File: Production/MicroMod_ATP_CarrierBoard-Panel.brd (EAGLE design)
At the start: 200.9 x 126 mm, 877 parts, among them J19 QWIIC_RIGHT_ANGLE, J2 JTAG, J20 QWIIC_RIGHT_ANGLE, J21 1X04_SMD_STRAIGHT_COMBO, J27 MICROMOD-2222-C, J28 USB_A_SMT_FEMALE, J34 QWIIC_RIGHT_ANGLE, J35 QWIIC_RIGHT_ANGLE, J37 1X04_SMD_STRAIGHT_COMBO, J4 USB_A_SMT_FEMALE, J40 1X04_SMD_STRAIGHT_COMBO, J50 JTAG, J51 MICROMOD-2222-C, J52 USB_A_SMT_FEMALE, J58 QWIIC_RIGHT_ANGLE, J59 QWIIC_RIGHT_ANGLE, J6 MICROMOD-2222-C, J61 1X04_SMD_STRAIGHT_COMBO, J64 1X04_SMD_STRAIGHT_COMBO, J7 JTAG, J74 JTAG, J75 MICROMOD-2222-C, J76 USB_A_SMT_FEMALE, J8 1X04_SMD_STRAIGHT_COMBO, J82 QWIIC_RIGHT_ANGLE, J83 QWIIC_RIGHT_ANGLE, J85 1X04_SMD_STRAIGHT_COMBO, J88 1X04_SMD_STRAIGHT_COMBO, U1 AP7361C-33, U2 AP7361C-33, U3 AP7361C-33, U5 AP7361C-33

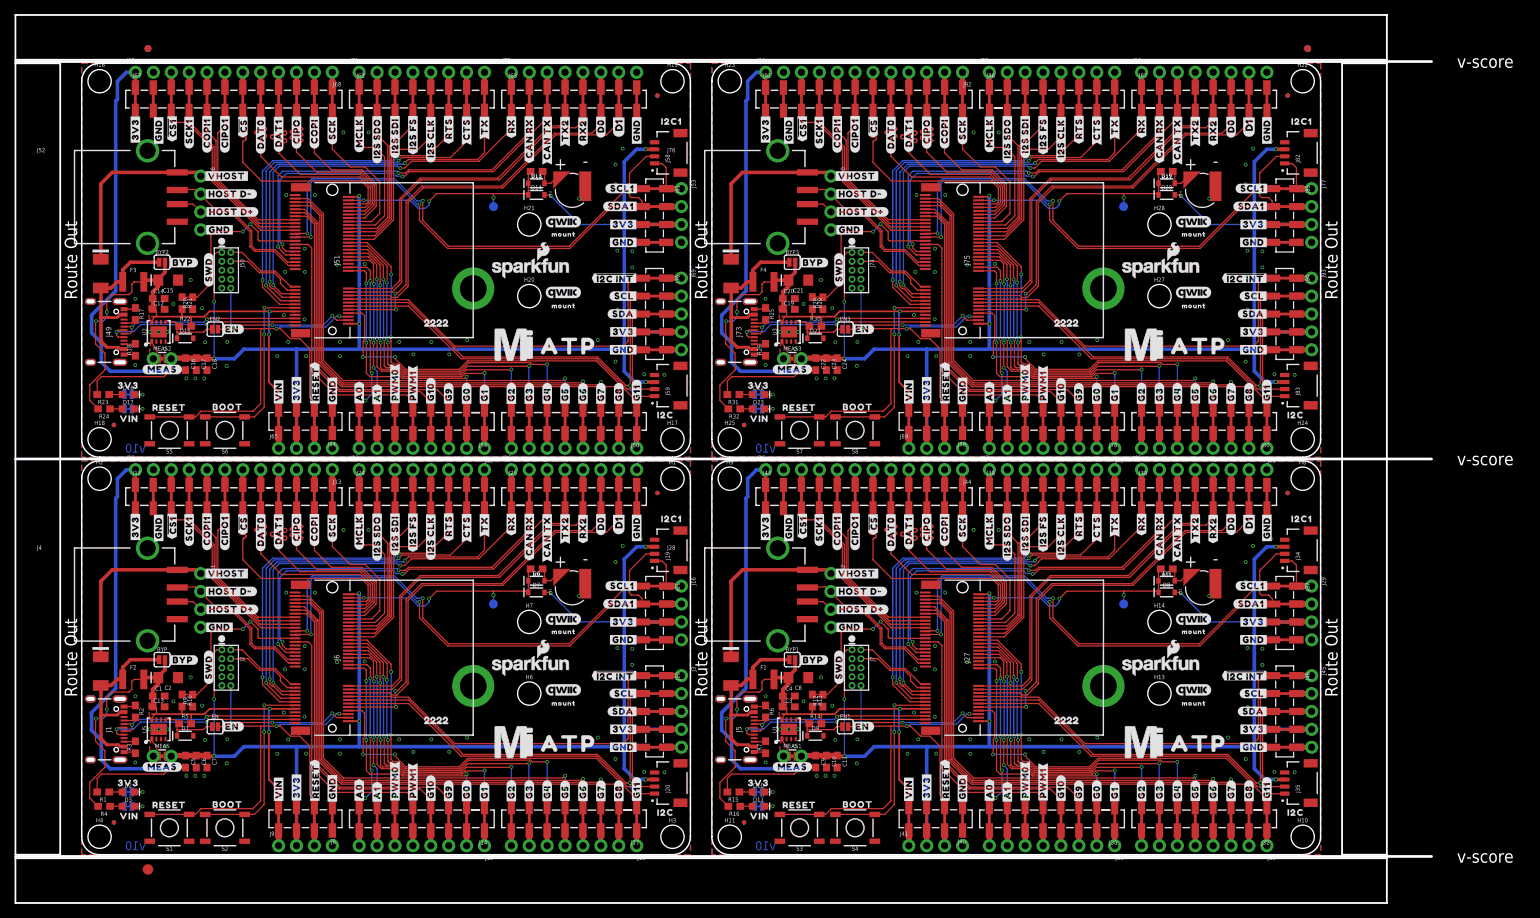
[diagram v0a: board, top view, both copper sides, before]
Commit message: Updates production files
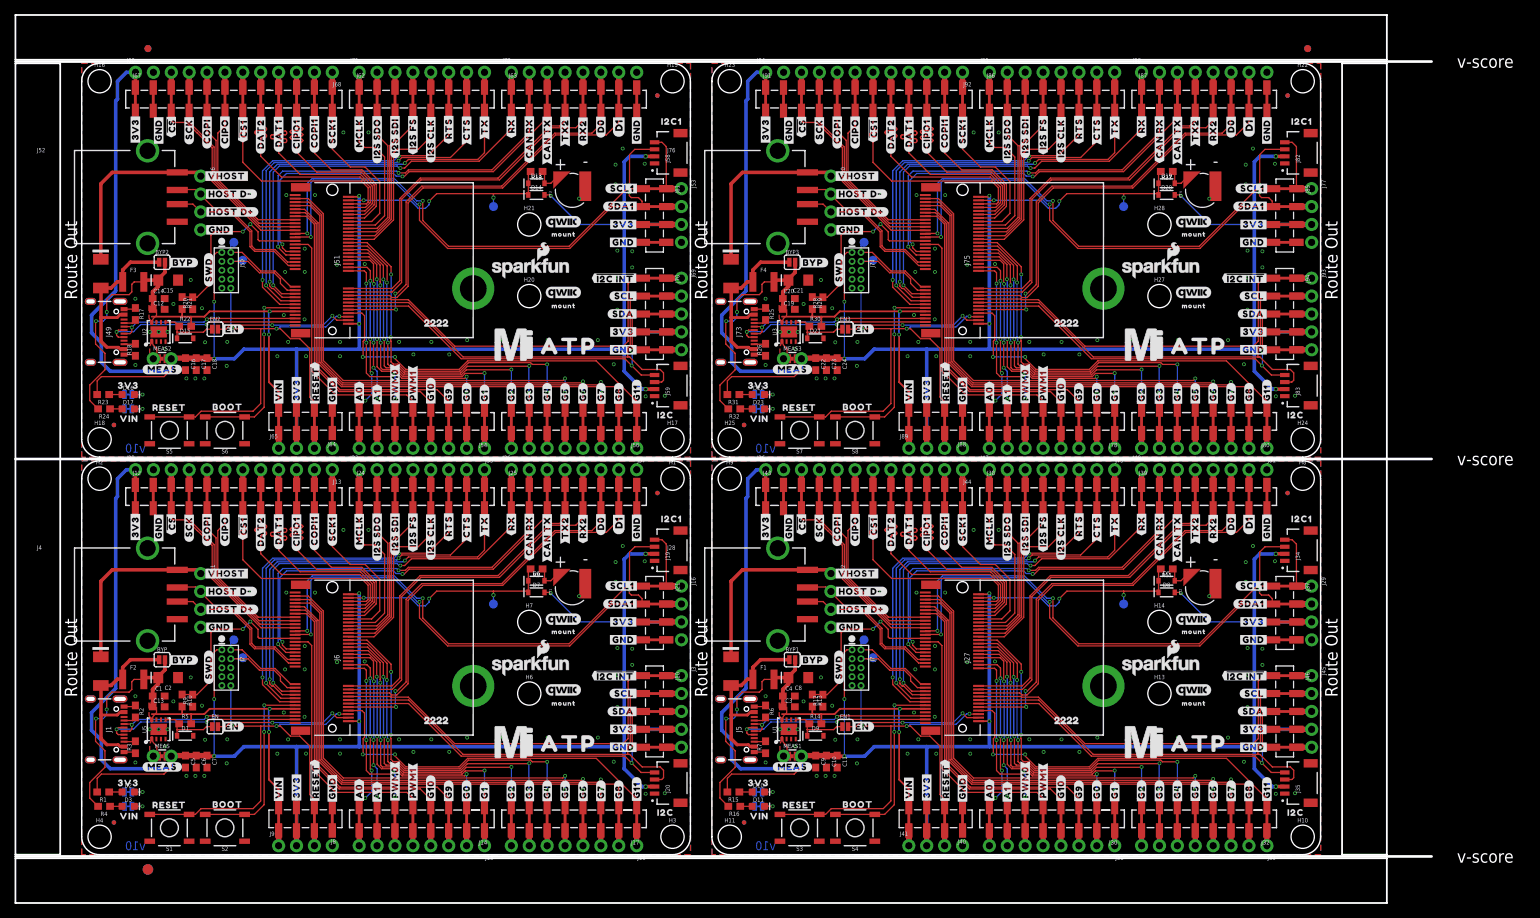
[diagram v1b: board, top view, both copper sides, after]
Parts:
- added E$6: (no value), SparkFun-Retired:FIDUCIAL-1.5X3
- added TP10, TP11, TP12, TP5, TP6, TP7, TP8, TP9: TEST-POINT3X5, SparkFun-Connectors:PAD.03X.05
- U$130: device buzzard_labels (9):22229 -> headtop:#CAN_RX#9
- U$147: device headtop:#CAN_RX#9 -> alc:#CIPO#5178038
- U$190, U$335, U$480: device headtop:#DAT1#4 -> headers_dup:#RX2#3
- U$191, U$336, U$481: device headtop:#DAT0#4 -> headers_dup:#TX2#2
- U$192, U$337, U$482: device headers_dup:#RX2#3 -> headers_dup:#SCL1#3
- U$193, U$338, U$483: device headers_dup:#TX2#2 -> headers_dup:#SDA1#3
- U$194, U$339, U$484: device headers_dup:#SCL1#3 -> headers_dup:#SCK1#2
- U$195, U$340, U$485: device headers_dup:#SDA1#3 -> headers_dup:VIN3
- U$196, U$341, U$486: device headers_dup:#SCK1#2 -> headers_dup:3V34
- U$197, U$342, U$487: device headers_dup:VIN3 -> power:#3V3#1
- U$198, U$343, U$488: device headers_dup:3V34 -> power:#3V3#1
- U$20: device headers_dup:##CS1##2 -> alc:##CS1##5178039
- U$201, U$346, U$491: device power:#3V3#1 -> headers_dup:ATP0
- U$202, U$347, U$492: device power:#3V3#1 -> headers_dup:I2C4
- U$203, U$348, U$493: device headers_dup:ATP0 -> headers_dup:I2C14
- U$204, U$349, U$494: device headers_dup:I2C4 -> headers_dup:ATP_CARRIER_BOARD1
- U$205, U$350, U$495: device headers_dup:I2C14 -> headers_dup:#COPI1#2
- U$206, U$351, U$496: device headers_dup:ATP_CARRIER_BOARD1 -> power:##RESET##7
- U$207, U$352, U$497: device fl1:##CS1##0 -> headtop:##CS##0
- U$208, U$353, U$498: device headers_dup:#CIPO1#2 -> fl1:#COPI1#2
- U$209, U$354, U$499: device headers_dup:#COPI1#2 -> fl1:#RX2#3
- U$210, U$355, U$500: device headers_dup:##CS1##2 -> fl1:#SCK1#2
- U$211, U$356, U$501: device power:##RESET##7 -> fl1:#SCL1#3
- U$212, U$357, U$502: device headtop:##CS##0 -> fl1:#SDA1#3
- U$213, U$358, U$503: device fl1:#CIPO1#2 -> fl1:#TX2#2
- U$214, U$359, U$504: device fl1:#COPI1#2 -> fl2:#DAT2#5
- U$215, U$360, U$505: device fl1:#RX2#3 -> fl2:#DAT1#5
- U$216, U$361, U$506: device fl1:#SCK1#2 -> fl2:#COPI#4
- U$217, U$362, U$507: device fl1:#SCL1#3 -> fl2:#SCK#4
- U$218, U$363, U$508: device fl1:#SDA1#3 -> fl2:#MCLK#6
- U$219, U$364, U$509: device fl1:#TX2#2 -> fl2:#I2S_FS#7
- U$220, U$365, U$510: device fl2:##CS##DAT3#0 -> fl2:#I2S_CLK#7
- U$221, U$366, U$511: device fl2:#DAT2#5 -> fl2:#RTS#7
- U$222, U$367, U$512: device fl2:#DAT1#5 -> fl2:#CTS#8
- U$223, U$368, U$513: device fl2:#COPI#4 -> fl2:#TX#9
- U$224, U$369, U$514: device fl2:#SCK#4 -> fl2:#RX#10
- U$225, U$370, U$515: device fl2:#MCLK#6 -> fl2:#CAN_RX#10
- U$226, U$371, U$516: device fl2:#I2S_FS#7 -> fl2:#CAN_TX#10
- U$227, U$372, U$517: device fl2:#I2S_CLK#7 -> fl4:#D0#0
- U$228, U$373, U$518: device fl2:#RTS#7 -> fl3:#GND#0
- U$229, U$374, U$519: device fl2:#CTS#8 -> fl3:#GND#0
- U$230, U$375, U$520: device fl2:#TX#9 -> fl3:#GND#0
- U$231, U$376, U$521: device fl2:#RX#10 -> fl3:#GND#0
- U$232, U$377, U$522: device fl2:#CAN_RX#10 -> fl3:#GND#0
- U$233, U$378, U$523: device fl2:#CAN_TX#10 -> fl3:#GND#0
- U$234, U$379, U$524: device fl4:#D0#0 -> fl3:#3V3#1
- U$235, U$380, U$525: device fl3:#GND#0 -> fl3:#3V3#1
- U$236, U$381, U$526: device fl3:#GND#0 -> fl3:#SDA#4
- U$237, U$382, U$527: device fl3:#GND#0 -> fl3:#SCL#5
- U$238, U$383, U$528: device fl3:#GND#0 -> fl2:##I2C_INT##10
- U$239, U$384, U$529: device fl3:#GND#0 -> fl4:#G11#10
- U$240, U$385, U$530: device fl3:#GND#0 -> fl4:#G8#8
- U$241, U$386, U$531: device fl3:#3V3#1 -> fl4:#G7#7
- U$242, U$387, U$532: device fl3:#3V3#1 -> fl4:#G6#6
- U$243, U$388, U$533: device fl3:#SDA#4 -> fl4:#G5#5
- U$244, U$389, U$534: device fl3:#SCL#5 -> fl4:#G4#4
- U$245, U$390, U$535: device fl2:##I2C_INT##10 -> fl4:#G3#3
- U$246, U$391, U$536: device fl4:#G11#10 -> fl4:#G2#2
- U$247, U$392, U$537: device fl4:#G8#8 -> fl4:#G1#2
- U$248, U$393, U$538: device fl4:#G7#7 -> fl4:#G0#2
- U$249, U$394, U$539: device fl4:#G6#6 -> fl4:#PWM0#10
- U$250, U$395, U$540: device fl4:#G5#5 -> fl4:#PWM1#10
- U$251, U$396, U$541: device fl4:#G4#4 -> fl4:#A0#10
- U$252, U$397, U$542: device fl4:#G3#3 -> fl4:#A1#10
- U$253, U$398, U$543: device fl4:#G2#2 -> fl3:##RESET##7
- U$254, U$399, U$544: device fl4:#G1#2 -> fl3:#3V3#1
- U$255, U$400, U$545: device fl4:#G0#2 -> fl3:#VIN#6
- U$256, U$401, U$546: device fl4:#PWM0#10 -> fl3:#HOST_D##9
- U$257, U$402, U$547: device fl4:#PWM1#10 -> fl3:#HOST_D##10
- U$258, U$403, U$548: device fl4:#A0#10 -> fl3:#SWD#10
- U$259, U$404, U$549: device fl4:#A1#10 -> fl3:#MEAS#10
- U$260, U$405, U$550: device fl3:##RESET##7 -> fl3:#VIN_LED#10
- U$261, U$406, U$551: device fl3:#3V3#1 -> fl3:#3V3_LED#10
- U$262, U$407, U$552: device fl3:#VIN#6 -> fl4:#G9#ADC##CAM_HSYNC#9
- U$263, U$408, U$553: device fl3:#HOST_D##9 -> fl4:#G10#ADC##CAM_VSYNC#10
- U$264, U$409, U$554: device fl3:#HOST_D##10 -> fl2:#I2S_SDI#CAM_PCLK#7
- U$265, U$410, U$555: device fl3:#SWD#10 -> fl2:#I2S_SDO#CAM_MCLK#7
- U$266, U$411, U$556: device fl3:#MEAS#10 -> fl3:#3V3#1
- U$267, U$412, U$557: device fl3:#VIN_LED#10 -> headtop:#SCK#2
- U$268, U$413, U$558: device fl3:#3V3_LED#10 -> power:#GND#0
- U$269, U$414, U$559: device fl4:#G9#ADC##CAM_HSYNC#9 -> power:#GND#0
- U$270, U$415, U$560: device fl4:#G10#ADC##CAM_VSYNC#10 -> power:#GND#0
- U$271, U$416, U$561: device fl2:#I2S_SDI#CAM_PCLK#7 -> headtop:##I2C_INT##10
- U$272, U$417, U$562: device fl2:#I2S_SDO#CAM_MCLK#7 -> D1:D10
- U$273, U$418, U$563: device fl3:#3V3#1 -> SparkFun-MicroMod:MICROMOD_MI_LOGO_1
- U$274, U$419, U$564: device headtop:#SCK#2 -> headtop:MOUNT10
- U$275, U$276, U$277, U$420, U$421, U$422, U$565, U$566, U$567: device power:#GND#0 -> headtop:MOUNT10
- U$278, U$423, U$568: device headtop:##I2C_INT##10 -> SparkFun-MicroMod:MICROMOD_LOGO_1
- U$279, U$424, U$569: device D1:D10 -> D1_again:D10
- U$280, U$425, U$570: device SparkFun-MicroMod:MICROMOD_MI_LOGO_1 -> output:#EN#0
- U$281, U$282, U$426, U$427, U$571, U$572: device headtop:MOUNT10 -> output:#VHOST#0
- U$283, U$428, U$573: device headtop:MOUNT10 -> alc:##CS##5178037
- U$284, U$429, U$574: device headtop:MOUNT10 -> alc:##CS1##DAT3#5178037
- U$285, U$430, U$575: device SparkFun-MicroMod:MICROMOD_LOGO_1 -> alc:#CIPO#5178038
- U$286, U$431, U$576: device fl2:#CIPO#DAT0#6 -> alc:##CS1##5178039
- U$287, U$432, U$577: device D1_again:D10 -> alc:#DAT1#5178039
- U$288, U$433, U$578: device output:#EN#0 -> alc:#DAT2#5178039
- U$289, U$434, U$579: device output:#VHOST#0 -> alc:#CIPO1#5178039
- U$290, U$435, U$580: device output:#VHOST#0 -> alc:##CIPO1##DAT0#5178038
- U$36: device fl1:##CS1##0 -> alc:#DAT1#5178039
- U$53: device headtop:#DAT1#4 -> alc:#DAT2#5178039
- U$54: device headtop:#DAT0#4 -> alc:#CIPO1#5178039
- U$56: device headers_dup:#CIPO1#2 -> alc:##CIPO1##DAT0#5178038
- U$74: device fl1:#CIPO1#2 -> buzzard_labels (9):22229
- U$81: device fl2:##CS##DAT3#0 -> alc:##CS##5178037
- U$84: device fl2:#CIPO#DAT0#6 -> alc:##CS1##DAT3#5178037
- moved U$147 132.7 mm to (20.3, 51.7), flipped to the bottom, turned to 270 degrees
- moved TP2 126.3 mm to (21.6, 30.5)
- moved U$74 121.1 mm to (137.0, 19.1), flipped to the top, turned to 0 degrees
- moved U$347 85.4 mm to (82.8, 62.4), turned to 0 degrees
- moved U$202 85.4 mm to (172.2, 5.97), turned to 0 degrees
- moved U$492 85.4 mm to (172.2, 62.4), turned to 0 degrees
- moved U$239 83.9 mm to (168.1, 3.56)
- moved U$384 83.9 mm to (78.7, 59.9)
- moved U$529 83.9 mm to (168.1, 59.9)
- moved U$195 76.0 mm to (96.1, 5.46)
- moved U$340 76.0 mm to (6.73, 61.8)
- moved U$485 76.0 mm to (96.1, 61.8)
- moved U$200 74.9 mm to (97.0, 46.5), turned to 90 degrees
- moved U$345 74.9 mm to (7.62, 102.9), turned to 90 degrees
- moved U$490 74.9 mm to (97.0, 102.9), turned to 90 degrees
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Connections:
- net !CS!/DAT1 renamed !CS1!/DAT1
- net !CS!/DAT2 renamed !CS1!/DAT2
- net !CS!/DAT3 renamed !CS1!/DAT3
- net !CS!/DAT4 renamed !CS1!/DAT4
- net !CS1 renamed !CS!
- net !CS2 renamed !CS!1
- net !CS3 renamed !CS!2
- net !CS4 renamed !CS!3
- net CIPO/DAT0 renamed CIPO1/DAT0
- net CIPO/DAT1 renamed CIPO1/DAT1
- net CIPO/DAT2 renamed CIPO1/DAT2
- net CIPO/DAT3 renamed CIPO1/DAT3
- removed net CIPO4: J75.61, J91.6, J92.7
- new net CIPO: J12.6, J13.7, J6.61
- net 3.3V: now also J19.2, J20.2; no longer J19.3, J20.3
- net 3.3V1: now also J34.2, J35.2; no longer J34.3, J35.3
- net 3.3V2: now also J58.2, J59.2; no longer J58.3, J59.3
- net 3.3V3: now also J82.2, J83.2; no longer J82.3, J83.3
- net CIPO1: now also J27.61, J43.6, J44.7; no longer J12.6, J13.7, J6.61
- net CIPO2: now also J51.61, J67.6, J68.7; no longer J27.61, J43.6, J44.7
- net CIPO3: now also J75.61, J91.6, J92.7; no longer J51.61, J67.6, J68.7
- net COPI: now also J12.5, J13.8, J6.59; no longer J12.11, J13.2, J6.62
- net COPI1: now also J12.11, J13.2, J6.62; no longer J12.5, J13.8, J6.59
- net COPI2: now also J27.59, J43.5, J44.8; no longer J27.62, J43.11, J44.2
- net COPI3: now also J27.62, J43.11, J44.2; no longer J27.59, J43.5, J44.8
- net COPI4: now also J51.59, J67.5, J68.8; no longer J51.62, J67.11, J68.2
- net COPI5: now also J51.62, J67.11, J68.2; no longer J51.59, J67.5, J68.8
- net COPI6: now also J75.59, J91.5, J92.8; no longer J75.62, J91.11, J92.2
- net COPI7: now also J75.62, J91.11, J92.2; no longer J75.59, J91.5, J92.8
- net GND: now also J19.1, J20.1; no longer J19.4, J20.4
- net GND1: now also J34.1, J35.1; no longer J34.4, J35.4
- net GND2: now also J58.1, J59.1; no longer J58.4, J59.4
- net GND3: now also J82.1, J83.1; no longer J82.4, J83.4
- net RTC_3V1: now also TP4.P$1; no longer TP2.P$1
- net RTC_3V2: now also TP7.P$1; no longer TP3.P$1
- net RTC_3V3: now also TP10.P$1; no longer TP4.P$1
- net SCK: now also J12.4, J22.4, J6.57; no longer J12.12, J13.1, J6.60
- net SCK1: now also J12.12, J13.1, J6.60; no longer J12.4, J22.4, J6.57
- net SCK2: now also J27.57, J36.4, J43.4; no longer J27.60, J43.12, J44.1
- net SCK3: now also J27.60, J43.12, J44.1; no longer J27.57, J36.4, J43.4
- net SCK4: now also J51.57, J60.4, J67.4; no longer J51.60, J67.12, J68.1
- net SCK5: now also J51.60, J67.12, J68.1; no longer J51.57, J60.4, J67.4
- net SCK6: now also J75.57, J84.4, J91.4; no longer J75.60, J91.12, J92.1
- net SCK7: now also J75.60, J91.12, J92.1; no longer J75.57, J84.4, J91.4
- net SCL: now also J20.3; no longer J20.1
- net SCL1: now also J19.4; no longer J19.1
- net SCL2: now also J35.3; no longer J35.1
- net SCL3: now also J34.4; no longer J34.1
- net SCL4: now also J59.3; no longer J59.1
- net SCL5: now also J58.4; no longer J58.1
- net SCL6: now also J83.3; no longer J83.1
- net SCL7: now also J82.4; no longer J82.1
- net SDA: now also J20.4; no longer J20.2
- net SDA1: now also J19.3; no longer J19.2
- net SDA2: now also J35.4; no longer J35.2
- net SDA3: now also J34.3; no longer J34.2
- net SDA4: now also J59.4; no longer J59.2
- net SDA5: now also J58.3; no longer J58.2
- net SDA6: now also J83.4; no longer J83.2
- net SDA7: now also J82.3; no longer J82.2
- net SWDCK: now also TP3.P$1
- net SWDCK1: now also TP6.P$1
- net SWDCK2: now also TP9.P$1
- net SWDCK3: now also TP12.P$1
- net SWDIO: now also TP2.P$1
- net SWDIO1: now also TP5.P$1
- net SWDIO2: now also TP8.P$1
- net SWDIO3: now also TP11.P$1
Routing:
- net CIPO: track 0.00 -> 29.0 mm
- net CIPO4: track 29.0 -> 0.00 mm
- net SDA2: track 65.9 -> 61.6 mm, vias 0 -> 2
- net SDA: track 65.9 -> 61.6 mm, vias 0 -> 2
- net SDA4: track 65.9 -> 61.6 mm, vias 0 -> 2
- net SDA6: track 65.9 -> 61.6 mm, vias 0 -> 2
- net SCL1: track 78.3 -> 81.3 mm
- net SCL7: track 78.3 -> 81.3 mm
- net SCL5: track 78.3 -> 81.3 mm
- net SCL3: track 78.3 -> 81.3 mm
- net COPI7: track 29.6 -> 32.0 mm
- net COPI6: track 32.0 -> 29.6 mm
- net COPI5: track 29.6 -> 32.0 mm
- net COPI3: track 29.6 -> 32.0 mm
- net COPI2: track 32.0 -> 29.6 mm
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
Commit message: Revert "Updates production files"
This reverts commit 213e6b1cbeb41024665e9e154624d95cc9d0b3ef.
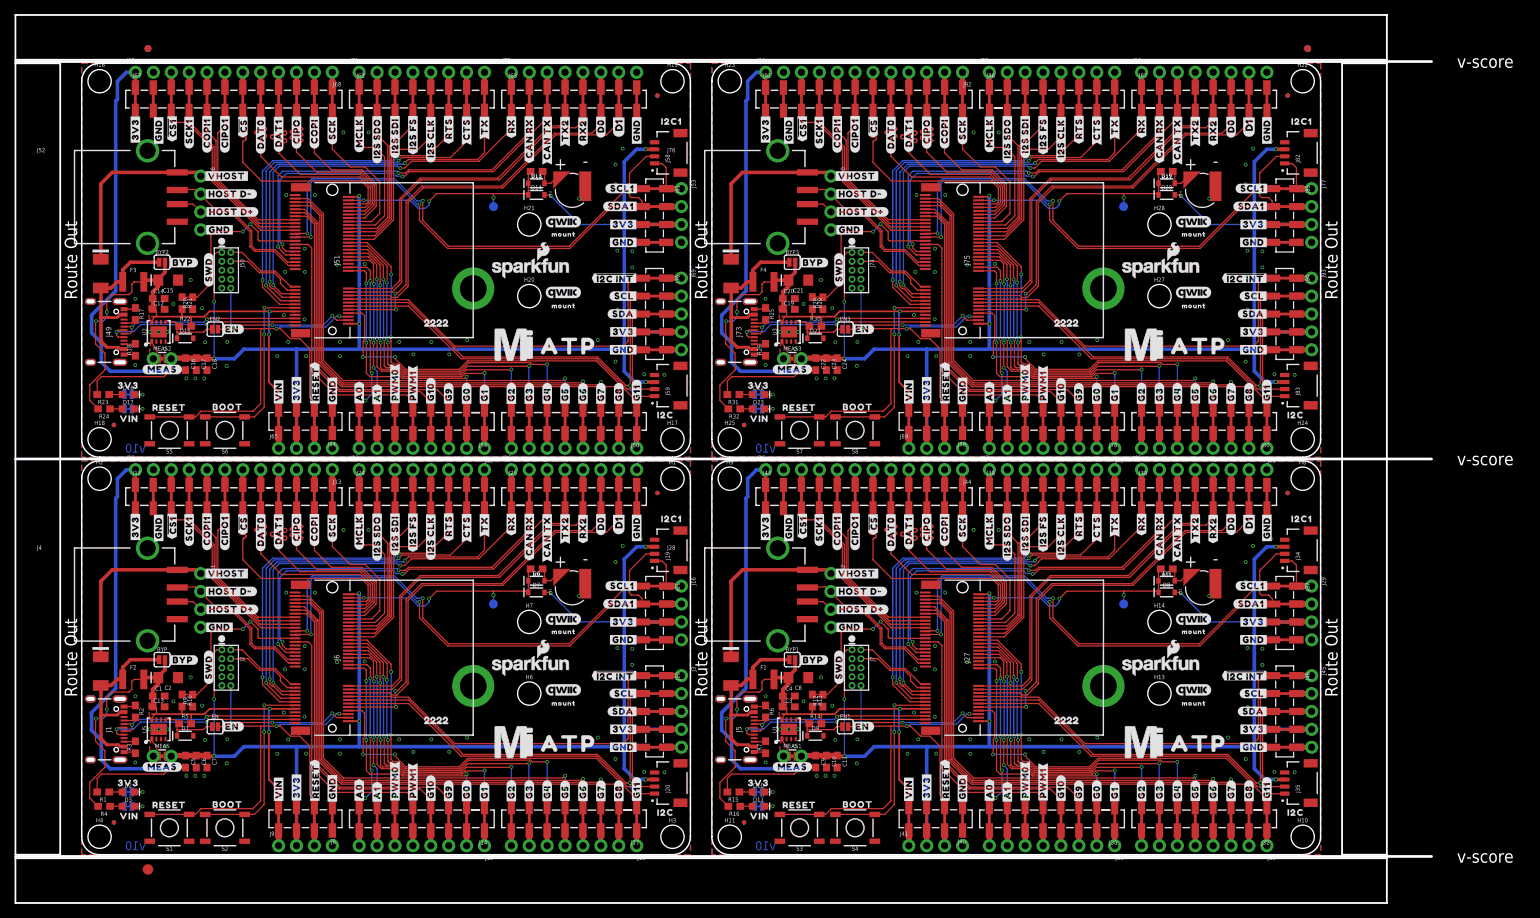
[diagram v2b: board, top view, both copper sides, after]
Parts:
- removed E$6: (no value), SparkFun-Retired:FIDUCIAL-1.5X3
- removed TP10, TP11, TP12, TP5, TP6, TP7, TP8, TP9: TEST-POINT3X5, SparkFun-Connectors:PAD.03X.05
- U$130: device headtop:#CAN_RX#9 -> buzzard_labels (9):22229
- U$147: device alc:#CIPO#5178038 -> headtop:#CAN_RX#9
- U$190, U$335, U$480: device headers_dup:#RX2#3 -> headtop:#DAT1#4
- U$191, U$336, U$481: device headers_dup:#TX2#2 -> headtop:#DAT0#4
- U$192, U$337, U$482: device headers_dup:#SCL1#3 -> headers_dup:#RX2#3
- U$193, U$338, U$483: device headers_dup:#SDA1#3 -> headers_dup:#TX2#2
- U$194, U$339, U$484: device headers_dup:#SCK1#2 -> headers_dup:#SCL1#3
- U$195, U$340, U$485: device headers_dup:VIN3 -> headers_dup:#SDA1#3
- U$196, U$341, U$486: device headers_dup:3V34 -> headers_dup:#SCK1#2
- U$197, U$342, U$487: device power:#3V3#1 -> headers_dup:VIN3
- U$198, U$343, U$488: device power:#3V3#1 -> headers_dup:3V34
- U$20: device alc:##CS1##5178039 -> headers_dup:##CS1##2
- U$201, U$346, U$491: device headers_dup:ATP0 -> power:#3V3#1
- U$202, U$347, U$492: device headers_dup:I2C4 -> power:#3V3#1
- U$203, U$348, U$493: device headers_dup:I2C14 -> headers_dup:ATP0
- U$204, U$349, U$494: device headers_dup:ATP_CARRIER_BOARD1 -> headers_dup:I2C4
- U$205, U$350, U$495: device headers_dup:#COPI1#2 -> headers_dup:I2C14
- U$206, U$351, U$496: device power:##RESET##7 -> headers_dup:ATP_CARRIER_BOARD1
- U$207, U$352, U$497: device headtop:##CS##0 -> fl1:##CS1##0
- U$208, U$353, U$498: device fl1:#COPI1#2 -> headers_dup:#CIPO1#2
- U$209, U$354, U$499: device fl1:#RX2#3 -> headers_dup:#COPI1#2
- U$210, U$355, U$500: device fl1:#SCK1#2 -> headers_dup:##CS1##2
- U$211, U$356, U$501: device fl1:#SCL1#3 -> power:##RESET##7
- U$212, U$357, U$502: device fl1:#SDA1#3 -> headtop:##CS##0
- U$213, U$358, U$503: device fl1:#TX2#2 -> fl1:#CIPO1#2
- U$214, U$359, U$504: device fl2:#DAT2#5 -> fl1:#COPI1#2
- U$215, U$360, U$505: device fl2:#DAT1#5 -> fl1:#RX2#3
- U$216, U$361, U$506: device fl2:#COPI#4 -> fl1:#SCK1#2
- U$217, U$362, U$507: device fl2:#SCK#4 -> fl1:#SCL1#3
- U$218, U$363, U$508: device fl2:#MCLK#6 -> fl1:#SDA1#3
- U$219, U$364, U$509: device fl2:#I2S_FS#7 -> fl1:#TX2#2
- U$220, U$365, U$510: device fl2:#I2S_CLK#7 -> fl2:##CS##DAT3#0
- U$221, U$366, U$511: device fl2:#RTS#7 -> fl2:#DAT2#5
- U$222, U$367, U$512: device fl2:#CTS#8 -> fl2:#DAT1#5
- U$223, U$368, U$513: device fl2:#TX#9 -> fl2:#COPI#4
- U$224, U$369, U$514: device fl2:#RX#10 -> fl2:#SCK#4
- U$225, U$370, U$515: device fl2:#CAN_RX#10 -> fl2:#MCLK#6
- U$226, U$371, U$516: device fl2:#CAN_TX#10 -> fl2:#I2S_FS#7
- U$227, U$372, U$517: device fl4:#D0#0 -> fl2:#I2S_CLK#7
- U$228, U$373, U$518: device fl3:#GND#0 -> fl2:#RTS#7
- U$229, U$374, U$519: device fl3:#GND#0 -> fl2:#CTS#8
- U$230, U$375, U$520: device fl3:#GND#0 -> fl2:#TX#9
- U$231, U$376, U$521: device fl3:#GND#0 -> fl2:#RX#10
- U$232, U$377, U$522: device fl3:#GND#0 -> fl2:#CAN_RX#10
- U$233, U$378, U$523: device fl3:#GND#0 -> fl2:#CAN_TX#10
- U$234, U$379, U$524: device fl3:#3V3#1 -> fl4:#D0#0
- U$235, U$380, U$525: device fl3:#3V3#1 -> fl3:#GND#0
- U$236, U$381, U$526: device fl3:#SDA#4 -> fl3:#GND#0
- U$237, U$382, U$527: device fl3:#SCL#5 -> fl3:#GND#0
- U$238, U$383, U$528: device fl2:##I2C_INT##10 -> fl3:#GND#0
- U$239, U$384, U$529: device fl4:#G11#10 -> fl3:#GND#0
- U$240, U$385, U$530: device fl4:#G8#8 -> fl3:#GND#0
- U$241, U$386, U$531: device fl4:#G7#7 -> fl3:#3V3#1
- U$242, U$387, U$532: device fl4:#G6#6 -> fl3:#3V3#1
- U$243, U$388, U$533: device fl4:#G5#5 -> fl3:#SDA#4
- U$244, U$389, U$534: device fl4:#G4#4 -> fl3:#SCL#5
- U$245, U$390, U$535: device fl4:#G3#3 -> fl2:##I2C_INT##10
- U$246, U$391, U$536: device fl4:#G2#2 -> fl4:#G11#10
- U$247, U$392, U$537: device fl4:#G1#2 -> fl4:#G8#8
- U$248, U$393, U$538: device fl4:#G0#2 -> fl4:#G7#7
- U$249, U$394, U$539: device fl4:#PWM0#10 -> fl4:#G6#6
- U$250, U$395, U$540: device fl4:#PWM1#10 -> fl4:#G5#5
- U$251, U$396, U$541: device fl4:#A0#10 -> fl4:#G4#4
- U$252, U$397, U$542: device fl4:#A1#10 -> fl4:#G3#3
- U$253, U$398, U$543: device fl3:##RESET##7 -> fl4:#G2#2
- U$254, U$399, U$544: device fl3:#3V3#1 -> fl4:#G1#2
- U$255, U$400, U$545: device fl3:#VIN#6 -> fl4:#G0#2
- U$256, U$401, U$546: device fl3:#HOST_D##9 -> fl4:#PWM0#10
- U$257, U$402, U$547: device fl3:#HOST_D##10 -> fl4:#PWM1#10
- U$258, U$403, U$548: device fl3:#SWD#10 -> fl4:#A0#10
- U$259, U$404, U$549: device fl3:#MEAS#10 -> fl4:#A1#10
- U$260, U$405, U$550: device fl3:#VIN_LED#10 -> fl3:##RESET##7
- U$261, U$406, U$551: device fl3:#3V3_LED#10 -> fl3:#3V3#1
- U$262, U$407, U$552: device fl4:#G9#ADC##CAM_HSYNC#9 -> fl3:#VIN#6
- U$263, U$408, U$553: device fl4:#G10#ADC##CAM_VSYNC#10 -> fl3:#HOST_D##9
- U$264, U$409, U$554: device fl2:#I2S_SDI#CAM_PCLK#7 -> fl3:#HOST_D##10
- U$265, U$410, U$555: device fl2:#I2S_SDO#CAM_MCLK#7 -> fl3:#SWD#10
- U$266, U$411, U$556: device fl3:#3V3#1 -> fl3:#MEAS#10
- U$267, U$412, U$557: device headtop:#SCK#2 -> fl3:#VIN_LED#10
- U$268, U$413, U$558: device power:#GND#0 -> fl3:#3V3_LED#10
- U$269, U$414, U$559: device power:#GND#0 -> fl4:#G9#ADC##CAM_HSYNC#9
- U$270, U$415, U$560: device power:#GND#0 -> fl4:#G10#ADC##CAM_VSYNC#10
- U$271, U$416, U$561: device headtop:##I2C_INT##10 -> fl2:#I2S_SDI#CAM_PCLK#7
- U$272, U$417, U$562: device D1:D10 -> fl2:#I2S_SDO#CAM_MCLK#7
- U$273, U$418, U$563: device SparkFun-MicroMod:MICROMOD_MI_LOGO_1 -> fl3:#3V3#1
- U$274, U$419, U$564: device headtop:MOUNT10 -> headtop:#SCK#2
- U$275, U$276, U$277, U$420, U$421, U$422, U$565, U$566, U$567: device headtop:MOUNT10 -> power:#GND#0
- U$278, U$423, U$568: device SparkFun-MicroMod:MICROMOD_LOGO_1 -> headtop:##I2C_INT##10
- U$279, U$424, U$569: device D1_again:D10 -> D1:D10
- U$280, U$425, U$570: device output:#EN#0 -> SparkFun-MicroMod:MICROMOD_MI_LOGO_1
- U$281, U$282, U$426, U$427, U$571, U$572: device output:#VHOST#0 -> headtop:MOUNT10
- U$283, U$428, U$573: device alc:##CS##5178037 -> headtop:MOUNT10
- U$284, U$429, U$574: device alc:##CS1##DAT3#5178037 -> headtop:MOUNT10
- U$285, U$430, U$575: device alc:#CIPO#5178038 -> SparkFun-MicroMod:MICROMOD_LOGO_1
- U$286, U$431, U$576: device alc:##CS1##5178039 -> fl2:#CIPO#DAT0#6
- U$287, U$432, U$577: device alc:#DAT1#5178039 -> D1_again:D10
- U$288, U$433, U$578: device alc:#DAT2#5178039 -> output:#EN#0
- U$289, U$434, U$579: device alc:#CIPO1#5178039 -> output:#VHOST#0
- U$290, U$435, U$580: device alc:##CIPO1##DAT0#5178038 -> output:#VHOST#0
- U$36: device alc:#DAT1#5178039 -> fl1:##CS1##0
- U$53: device alc:#DAT2#5178039 -> headtop:#DAT1#4
- U$54: device alc:#CIPO1#5178039 -> headtop:#DAT0#4
- U$56: device alc:##CIPO1##DAT0#5178038 -> headers_dup:#CIPO1#2
- U$74: device buzzard_labels (9):22229 -> fl1:#CIPO1#2
- U$81: device alc:##CS##5178037 -> fl2:##CS##DAT3#0
- U$84: device alc:##CS1##DAT3#5178037 -> fl2:#CIPO#DAT0#6
- moved U$147 132.7 mm to (152.9, 45.2), flipped to the top, turned to 90 degrees
- moved TP2 126.3 mm to (147.8, 35.6)
- moved U$74 121.1 mm to (20.3, 51.3), flipped to the bottom, turned to 270 degrees
- moved U$347 85.4 mm to (7.62, 102.9), turned to 90 degrees
- moved U$202 85.4 mm to (97.0, 46.5), turned to 90 degrees
- moved U$492 85.4 mm to (97.0, 102.9), turned to 90 degrees
- moved U$239 83.9 mm to (99.6, 51.9)
- moved U$384 83.9 mm to (10.2, 108.3)
- moved U$529 83.9 mm to (99.6, 108.3)
- moved U$195 76.0 mm to (165.9, 35.6)
- moved U$340 76.0 mm to (76.5, 92.0)
- moved U$485 76.0 mm to (165.9, 92.0)
- moved U$200 74.9 mm to (166.2, 17.8), turned to 0 degrees
- moved U$345 74.9 mm to (76.8, 74.2), turned to 0 degrees
- moved U$490 74.9 mm to (166.2, 74.2), turned to 0 degrees
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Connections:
- net !CS! renamed !CS1
- net !CS!1 renamed !CS2
- net !CS!2 renamed !CS3
- net !CS!3 renamed !CS4
- net !CS1!/DAT1 renamed !CS!/DAT1
- net !CS1!/DAT2 renamed !CS!/DAT2
- net !CS1!/DAT3 renamed !CS!/DAT3
- net !CS1!/DAT4 renamed !CS!/DAT4
- net CIPO1/DAT0 renamed CIPO/DAT0
- net CIPO1/DAT1 renamed CIPO/DAT1
- net CIPO1/DAT2 renamed CIPO/DAT2
- net CIPO1/DAT3 renamed CIPO/DAT3
- removed net CIPO: J12.6, J13.7, J6.61
- new net CIPO4: J75.61, J91.6, J92.7
- net 3.3V: now also J19.3, J20.3; no longer J19.2, J20.2
- net 3.3V1: now also J34.3, J35.3; no longer J34.2, J35.2
- net 3.3V2: now also J58.3, J59.3; no longer J58.2, J59.2
- net 3.3V3: now also J82.3, J83.3; no longer J82.2, J83.2
- net CIPO1: now also J12.6, J13.7, J6.61; no longer J27.61, J43.6, J44.7
- net CIPO2: now also J27.61, J43.6, J44.7; no longer J51.61, J67.6, J68.7
- net CIPO3: now also J51.61, J67.6, J68.7; no longer J75.61, J91.6, J92.7
- net COPI: now also J12.11, J13.2, J6.62; no longer J12.5, J13.8, J6.59
- net COPI1: now also J12.5, J13.8, J6.59; no longer J12.11, J13.2, J6.62
- net COPI2: now also J27.62, J43.11, J44.2; no longer J27.59, J43.5, J44.8
- net COPI3: now also J27.59, J43.5, J44.8; no longer J27.62, J43.11, J44.2
- net COPI4: now also J51.62, J67.11, J68.2; no longer J51.59, J67.5, J68.8
- net COPI5: now also J51.59, J67.5, J68.8; no longer J51.62, J67.11, J68.2
- net COPI6: now also J75.62, J91.11, J92.2; no longer J75.59, J91.5, J92.8
- net COPI7: now also J75.59, J91.5, J92.8; no longer J75.62, J91.11, J92.2
- net GND: now also J19.4, J20.4; no longer J19.1, J20.1
- net GND1: now also J34.4, J35.4; no longer J34.1, J35.1
- net GND2: now also J58.4, J59.4; no longer J58.1, J59.1
- net GND3: now also J82.4, J83.4; no longer J82.1, J83.1
- net RTC_3V1: now also TP2.P$1; no longer TP4.P$1
- net RTC_3V2: now also TP3.P$1; no longer TP7.P$1
- net RTC_3V3: now also TP4.P$1; no longer TP10.P$1
- net SCK: now also J12.12, J13.1, J6.60; no longer J12.4, J22.4, J6.57
- net SCK1: now also J12.4, J22.4, J6.57; no longer J12.12, J13.1, J6.60
- net SCK2: now also J27.60, J43.12, J44.1; no longer J27.57, J36.4, J43.4
- net SCK3: now also J27.57, J36.4, J43.4; no longer J27.60, J43.12, J44.1
- net SCK4: now also J51.60, J67.12, J68.1; no longer J51.57, J60.4, J67.4
- net SCK5: now also J51.57, J60.4, J67.4; no longer J51.60, J67.12, J68.1
- net SCK6: now also J75.60, J91.12, J92.1; no longer J75.57, J84.4, J91.4
- net SCK7: now also J75.57, J84.4, J91.4; no longer J75.60, J91.12, J92.1
- net SCL: now also J20.1; no longer J20.3
- net SCL1: now also J19.1; no longer J19.4
- net SCL2: now also J35.1; no longer J35.3
- net SCL3: now also J34.1; no longer J34.4
- net SCL4: now also J59.1; no longer J59.3
- net SCL5: now also J58.1; no longer J58.4
- net SCL6: now also J83.1; no longer J83.3
- net SCL7: now also J82.1; no longer J82.4
- net SDA: now also J20.2; no longer J20.4
- net SDA1: now also J19.2; no longer J19.3
- net SDA2: now also J35.2; no longer J35.4
- net SDA3: now also J34.2; no longer J34.3
- net SDA4: now also J59.2; no longer J59.4
- net SDA5: now also J58.2; no longer J58.3
- net SDA6: now also J83.2; no longer J83.4
- net SDA7: now also J82.2; no longer J82.3
- net SWDCK: no longer TP3.P$1
- net SWDCK1: no longer TP6.P$1
- net SWDCK2: no longer TP9.P$1
- net SWDCK3: no longer TP12.P$1
- net SWDIO: no longer TP2.P$1
- net SWDIO1: no longer TP5.P$1
- net SWDIO2: no longer TP8.P$1
- net SWDIO3: no longer TP11.P$1
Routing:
- net CIPO: track 29.0 -> 0.00 mm
- net CIPO4: track 0.00 -> 29.0 mm
- net SDA2: track 61.6 -> 65.9 mm, vias 2 -> 0
- net SDA: track 61.6 -> 65.9 mm, vias 2 -> 0
- net SDA4: track 61.6 -> 65.9 mm, vias 2 -> 0
- net SDA6: track 61.6 -> 65.9 mm, vias 2 -> 0
- net SCL1: track 81.3 -> 78.3 mm
- net SCL7: track 81.3 -> 78.3 mm
- net SCL5: track 81.3 -> 78.3 mm
- net SCL3: track 81.3 -> 78.3 mm
- net COPI7: track 32.0 -> 29.6 mm
- net COPI6: track 29.6 -> 32.0 mm
- net COPI5: track 32.0 -> 29.6 mm
- net COPI3: track 32.0 -> 29.6 mm
- net COPI2: track 29.6 -> 32.0 mm
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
